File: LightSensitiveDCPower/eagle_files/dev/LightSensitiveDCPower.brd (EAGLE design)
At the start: 12 x 17.5 mm, 5 parts, among them SW1 PCM12SMTR

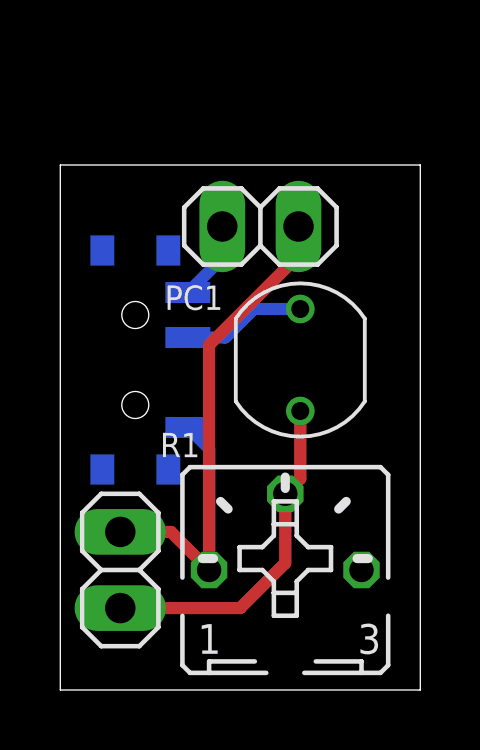
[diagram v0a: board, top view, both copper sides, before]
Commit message: Elongate board to save for wiidth. Check point.
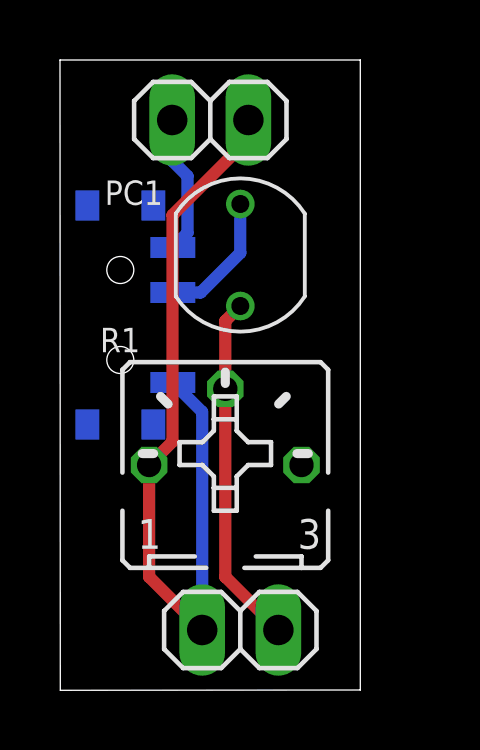
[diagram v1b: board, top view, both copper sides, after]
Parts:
- moved OUT 4.47 mm to (6.00, 2.00), turned to 0 degrees
- moved PC1 4.03 mm to (6.00, 14.5)
- moved R1 4.03 mm to (5.50, 7.50)
- moved IN 3.92 mm to (5.00, 19.0)
- moved SW1 1.58 mm to (2.00, 12.5)
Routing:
- net N$1: track 21.2 -> 27.8 mm
- net N$2: track 2.68 -> 4.66 mm
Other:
- board size 12 x 17.5 mm -> 10 x 21 mm
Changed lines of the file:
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@@
 <layer number="37" name="tTest" color="7" fill="1" visible="no" active="yes"/>
 <layer number="38" name="bTest" color="7" fill="1" visible="no" active="yes"/>
-<layer number="39" name="tKeepout" color="4" fill="11" visible="no" active="yes"/>
+<layer number="39" name="tKeepout" color="4" fill="11" visible="yes" active="yes"/>
 <layer number="40" name="bKeepout" color="1" fill="11" visible="yes" active="yes"/>
 <layer number="41" name="tRestrict" color="4" fill="10" visible="yes" active="yes"/>
@@
 <board>
 <plain>
-<wire x1="0" y1="0" x2="12" y2="0" width="0" layer="20"/>
-<wire x1="12" y1="0" x2="12" y2="17.5" width="0" layer="20"/>
-<wire x1="12" y1="17.5" x2="0" y2="17.5" width="0" layer="20"/>
-<wire x1="0" y1="17.5" x2="0" y2="0" width="0" layer="20"/>
-<text x="2" y="15.25" size="0.6096" layer="51">VIN</text>
-<text x="1.25" y="0.5" size="0.6096" layer="51">VOUT</text>
-<text x="1.25" y="7" size="0.6096" layer="51">GND</text>
-<text x="10" y="15.25" size="0.6096" layer="51">GND</text>
-<text x="1.46" y="10.41" size="0.3048" layer="51">LiSePow
+<wire x1="0" y1="-0.01" x2="10" y2="0" width="0" layer="20"/>
+<wire x1="10" y1="0" x2="10" y2="21" width="0" layer="20"/>
+<wire x1="10" y1="21" x2="-0.01" y2="21" width="0" layer="20"/>
+<wire x1="-0.01" y1="21" x2="0" y2="-0.01" width="0" layer="20"/>
+<text x="0.7" y="18.5" size="0.6096" layer="51">VIN</text>
+<text x="9.49" y="0.88" size="0.6096" layer="51" rot="R90">VOUT</text>
+<text x="2.77" y="1.16" size="0.6096" layer="51" rot="R90">GND</text>
+<text x="8" y="18.5" size="0.6096" layer="51">GND</text>
+<text x="1.31" y="12.87" size="0.3048" layer="51">LiSePow
 Rev1
 09/19/14</text>
@@
 </autorouter>
 <elements>
-<element name="IN" library="pinhead" package="1X02" value="" x="6.67" y="15.45" smashed="yes" rot="R180">
-<attribute name="VALUE" x="9.21" y="18.625" size="1.27" layer="27" rot="R180"/>
-</element>
-<element name="OUT" library="pinhead" package="1X02" value="" x="2" y="4" smashed="yes" rot="R270">
-<attribute name="VALUE" x="-1.175" y="6.54" size="1.27" layer="27" rot="R270"/>
-</element>
-<element name="PC1" library="freddyLibr" package="PHOTOCELL_CERAMIC" value="" x="8" y="11" smashed="yes">
-<attribute name="NAME" x="3.48" y="12.67" size="0.8128" layer="25"/>
-</element>
-<element name="R1" library="pot" package="B25P" value="" x="7.5" y="4" smashed="yes">
-<attribute name="NAME" x="3.325" y="7.76" size="0.8128" layer="25" ratio="10"/>
-<attribute name="VALUE" x="4.3504" y="-1.08" size="1.27" layer="27" ratio="10"/>
-</element>
-<element name="SW1" library="freddyLibr" package="PCM12SMTR" value="PCM12SMTR" x="2.5" y="11" smashed="yes" rot="MR90">
-<attribute name="NAME" x="3.13" y="15.63" size="0.8128" layer="26" rot="MR0"/>
+<element name="IN" library="pinhead" package="1X02" value="" x="5" y="19" smashed="yes" rot="R180">
+<attribute name="VALUE" x="7.54" y="22.175" size="1.27" layer="27" rot="R180"/>
+</element>
+<element name="OUT" library="pinhead" package="1X02" value="" x="6" y="2" smashed="yes">
+<attribute name="VALUE" x="3.46" y="-1.175" size="1.27" layer="27"/>
+</element>
+<element name="PC1" library="freddyLibr" package="PHOTOCELL_CERAMIC" value="" x="6" y="14.5" smashed="yes">
+<attribute name="NAME" x="1.48" y="16.17" size="0.8128" layer="25"/>
+</element>
+<element name="R1" library="pot" package="B25P" value="" x="5.5" y="7.5" smashed="yes">
+<attribute name="NAME" x="1.325" y="11.26" size="0.8128" layer="25" ratio="10"/>
+<attribute name="VALUE" x="2.3504" y="2.42" size="1.27" layer="27" ratio="10"/>
+</element>
+<element name="SW1" library="freddyLibr" package="PCM12SMTR" value="PCM12SMTR" x="2" y="12.5" smashed="yes" rot="MR90">
+<attribute name="NAME" x="2.63" y="17.13" size="0.8128" layer="26" rot="MR0"/>
 </element>
 </elements>
@@
 <contactref element="R1" pad="A"/>
 <contactref element="OUT" pad="1"/>
-<wire x1="2" y1="5.27" x2="3.69" y2="5.27" width="0.4064" layer="1"/>
-<wire x1="3.69" y1="5.27" x2="4.96" y2="4" width="0.4064" layer="1"/>
-<wire x1="4.96" y1="4" x2="4.96" y2="8.04" width="0.4064" layer="16"/>
-<wire x1="4.96" y1="8.04" x2="4.25" y2="8.75" width="0.4064" layer="16"/>
-<wire x1="7.94" y1="15.45" x2="7.94" y2="14.48" width="0.4064" layer="1"/>
-<wire x1="7.94" y1="14.48" x2="4.96" y2="11.5" width="0.4064" layer="1"/>
-<wire x1="4.96" y1="11.5" x2="4.96" y2="4" width="0.4064" layer="1"/>
+<wire x1="2.96" y1="7.5" x2="2.96" y2="3.77" width="0.4064" layer="1"/>
+<wire x1="2.96" y1="3.77" x2="4.73" y2="2" width="0.4064" layer="1"/>
+<wire x1="4.73" y1="2" x2="4.73" y2="9.27" width="0.4064" layer="16"/>
+<wire x1="4.73" y1="9.27" x2="3.75" y2="10.25" width="0.4064" layer="16"/>
+<wire x1="6.27" y1="19" x2="6.27" y2="18.36" width="0.4064" layer="1"/>
+<wire x1="6.27" y1="18.36" x2="3.74" y2="15.83" width="0.4064" layer="1"/>
+<wire x1="3.74" y1="15.83" x2="3.74" y2="8.28" width="0.4064" layer="1"/>
+<wire x1="3.74" y1="8.28" x2="2.96" y2="7.5" width="0.4064" layer="1"/>
 </signal>
 <signal name="N$2">
 <contactref element="IN" pad="2"/>
 <contactref element="SW1" pad="3"/>
-<wire x1="5.4" y1="15.45" x2="5.4" y2="14.4" width="0.4064" layer="16"/>
-<wire x1="5.4" y1="14.4" x2="4.25" y2="13.25" width="0.4064" layer="16"/>
+<wire x1="3.73" y1="19" x2="3.73" y2="17.64" width="0.4064" layer="16"/>
+<wire x1="3.73" y1="17.64" x2="4.24" y2="17.13" width="0.4064" layer="16"/>
+<wire x1="4.24" y1="17.13" x2="4.24" y2="15.24" width="0.4064" layer="16"/>
+<wire x1="4.24" y1="15.24" x2="3.75" y2="14.75" width="0.4064" layer="16"/>
 </signal>
 <signal name="N$3">
 <contactref element="SW1" pad="2"/>
 <contactref element="PC1" pad="1"/>
-<wire x1="8" y1="12.7" x2="6.45" y2="12.7" width="0.4064" layer="16"/>
-<wire x1="6.45" y1="12.7" x2="5.5" y2="11.75" width="0.4064" layer="16"/>
-<wire x1="5.5" y1="11.75" x2="4.25" y2="11.75" width="0.4064" layer="16"/>
+<wire x1="6" y1="16.2" x2="6" y2="14.57" width="0.4064" layer="16"/>
+<wire x1="6" y1="14.57" x2="4.68" y2="13.25" width="0.4064" layer="16"/>
+<wire x1="4.68" y1="13.25" x2="3.75" y2="13.25" width="0.4064" layer="16"/>
 </signal>
 <signal name="N$4">
@@
 <contactref element="OUT" pad="2"/>
 <contactref element="PC1" pad="2"/>
-<wire x1="8" y1="9.3" x2="8" y2="7.04" width="0.4064" layer="1"/>
-<wire x1="8" y1="7.04" x2="7.5" y2="6.54" width="0.4064" layer="1"/>
-<wire x1="7.5" y1="6.54" x2="7.5" y2="4.23" width="0.4064" layer="1"/>
-<wire x1="7.5" y1="4.23" x2="6" y2="2.73" width="0.4064" layer="1"/>
-<wire x1="6" y1="2.73" x2="2" y2="2.73" width="0.4064" layer="1"/>
+<wire x1="5.5" y1="10.04" x2="5.5" y2="12.3" width="0.4064" layer="1"/>
+<wire x1="5.5" y1="12.3" x2="6" y2="12.8" width="0.4064" layer="1"/>
+<wire x1="5.5" y1="10.04" x2="5.5" y2="3.77" width="0.4064" layer="1"/>
+<wire x1="5.5" y1="3.77" x2="7.27" y2="2" width="0.4064" layer="1"/>
 </signal>
 </signals>
